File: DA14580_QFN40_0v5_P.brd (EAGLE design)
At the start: 91 x 72 mm, 52 parts, among them CON1 CON_TC2030-CTL-NL, CON2 CON_TC2030-CTL-NL, IC1 IC_MEMORY_8P_AT25XE011_SOP, IC2 74LVC1G00DBV, IC3 IC_LDO_XX1117_5, IC4 IC_MEMORY_8P_AT25XE011_SOP, IC5 IC_LDO_XX1117_5, IC6 74LVC1G00DBV, U1 DA14583-AT2, U2 DA14583-AT2, X1 SSW-114-02-S-S, X2 SSW-114-02-S-S, X3 SSW-114-02-S-S, X4 SSW-114-02-S-S

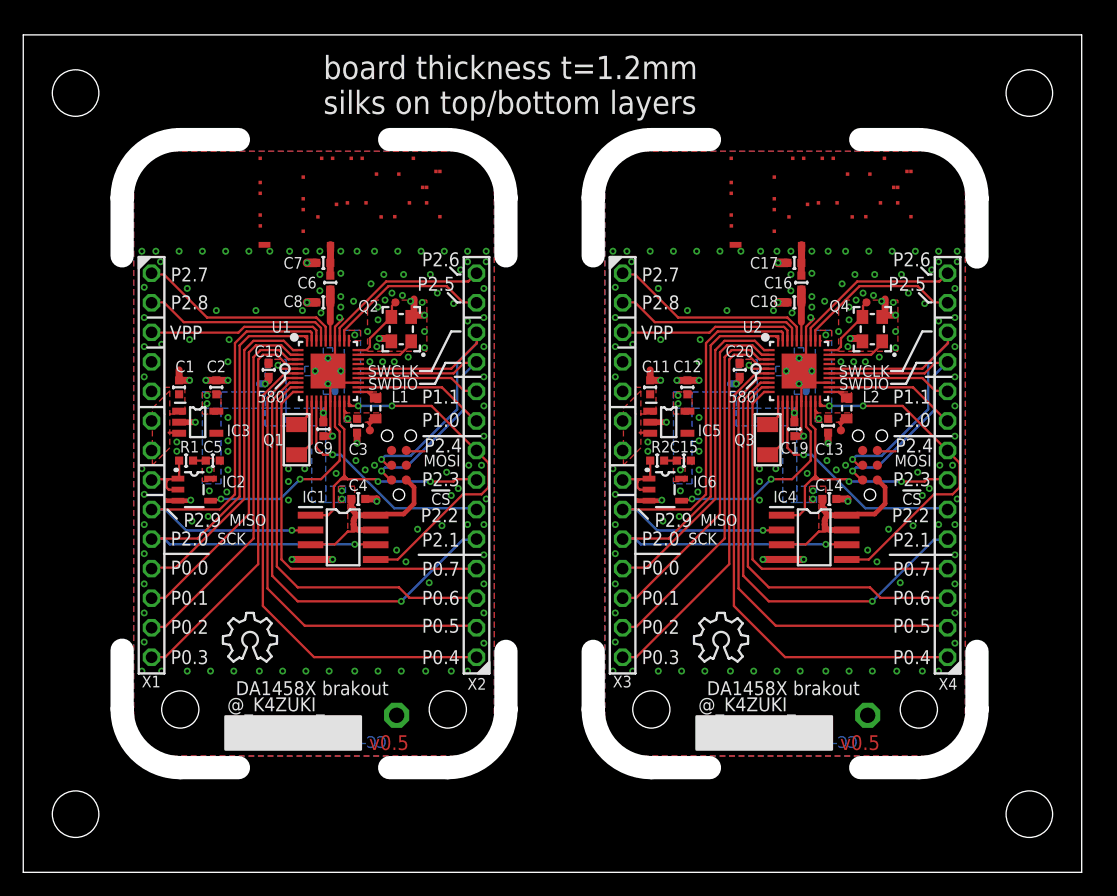
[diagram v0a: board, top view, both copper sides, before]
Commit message: [ 58x ] panelize and process gerber
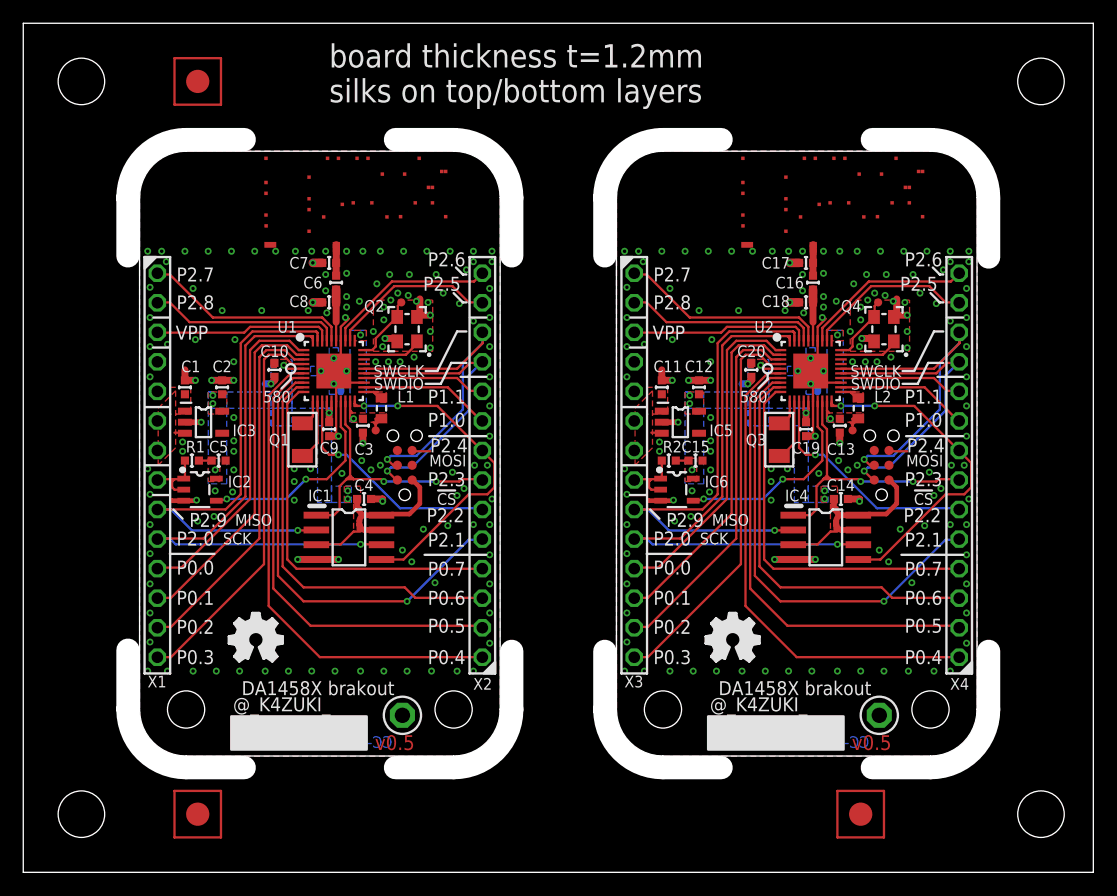
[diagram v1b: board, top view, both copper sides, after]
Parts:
- added TP7, TP8: TPTP07R, testpad_local:TP07R
- added TP9: TPPAD1-13, testpad_local:P1-13
- C16, C6: value (none) -> NM
- IC1, IC4: value IC_MEMORY_8P_AT25XE011_SOP -> 1265-1137-1-ND
- IC2, IC6: value 74LVC1G00DBV -> NC7SZ00M5XCT-ND
- L1, L2: value 2.2u -> (none)
- Q1, Q3: value (none) -> 728-1076-1-ND; device mylib:CR_3216 -> mylib:CRYSTAL_FC-135
- Q2, Q4: value (none) -> 887-1833-1-ND
- TP2, TP4: value TPTP07R -> TESTPAD_F; device testpad_local:TP07R -> mylib:FIDUCIAL
- TP5: value TPPAD1-13 -> TESTPAD_F; device testpad_local:P1-13 -> mylib:FIDUCIAL
- moved TP4 72.4 mm to (15.0, 5.00)
- moved TP2 62.9 mm to (15.0, 68.0)
- moved TP5 8.52 mm to (72.0, 5.00)
- moved C11 1.00 mm to (54.9, 41.7)
- moved C12 1.00 mm to (58.1, 41.7)
- moved C13 1.00 mm to (70.2, 38.4)
- moved C14 1.00 mm to (70.3, 32.1)
- moved C15 1.00 mm to (57.8, 35.4)
- moved C16 1.00 mm to (67.9, 50.7)
- moved C17 1.00 mm to (67.3, 52.4)
- moved C18 1.00 mm to (67.3, 49.0)
- moved C19 1.00 mm to (67.3, 38.1)
- moved C20 1.00 mm to (62.6, 43.2)
- moved CON2 1.00 mm to (73.8, 35.0)
- moved IC4 1.00 mm to (69.0, 28.8)
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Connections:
- net GND1: now also TP9.TP; no longer TP5.TP
- net N$5: now also TP8.TP; no longer TP4.TP
- net N$8: now also TP7.TP; no longer TP2.TP
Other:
- board size 91 x 72 mm -> 92 x 73 mm
